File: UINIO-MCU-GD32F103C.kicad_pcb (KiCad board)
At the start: 2 copper layers, 68.4 x 20.3 mm, 41 parts, among them J1 Conn_01x24_Pin, J2 Conn_01x24_Pin, J3 Conn_01x04_Pin, SW1 BOOT1, SW2 NRST, SW3 BOOT0, U1 ME6211C33M5G-N, U2 GD32F103C8T6, Y1 32.768KHz, Y2 8MHz

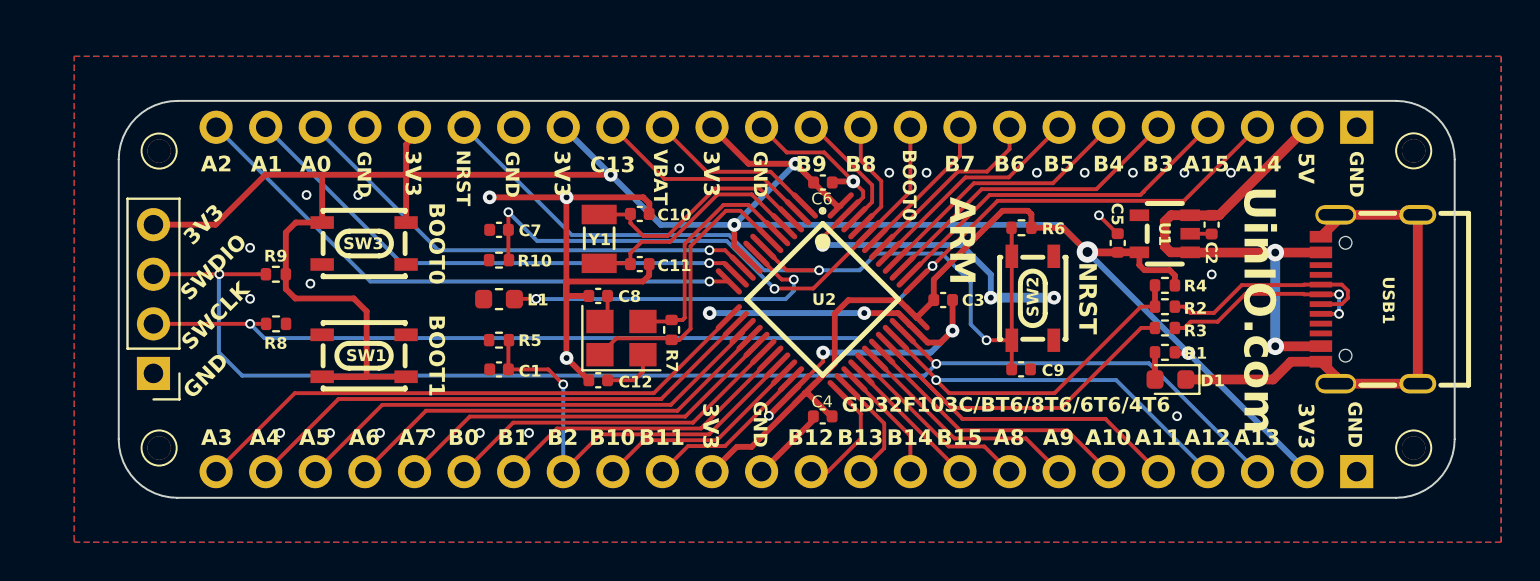
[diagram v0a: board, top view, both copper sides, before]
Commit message: Release UINIO-MCU-GD32F103C version 2.0.0.
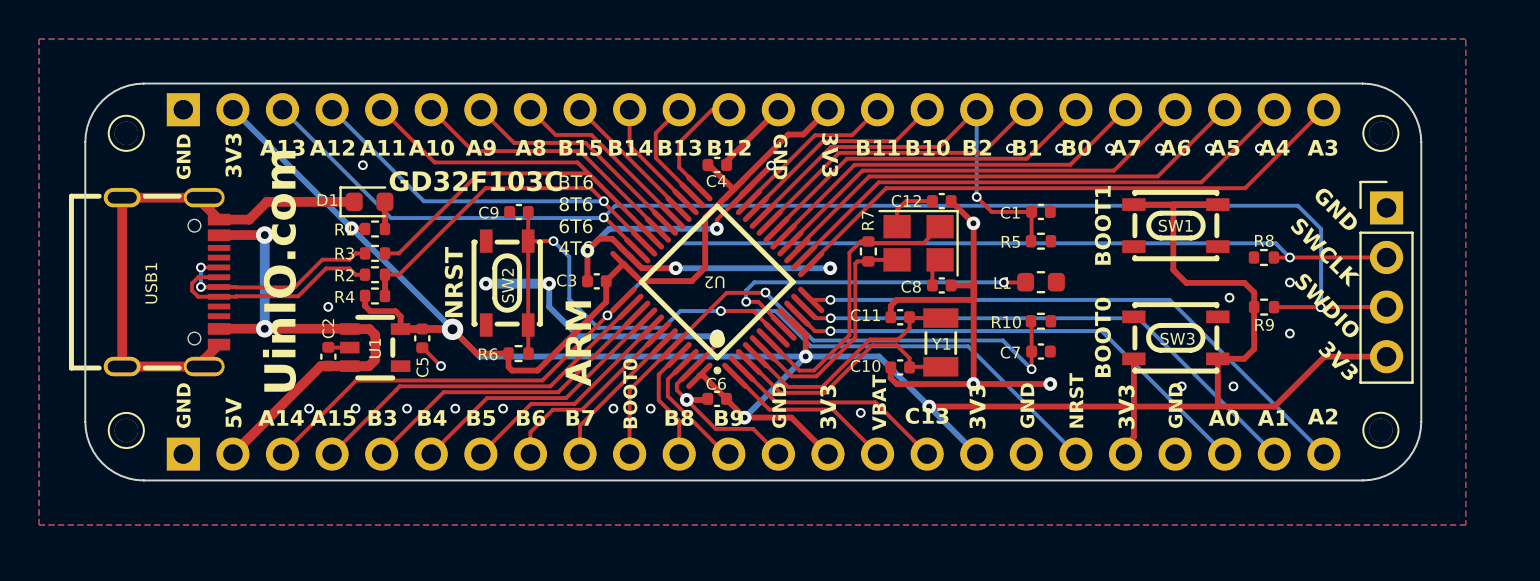
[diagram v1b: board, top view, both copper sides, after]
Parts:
- moved HOLE** 67.9 mm to (119.4, 92.2), turned to 180 degrees
- moved HOLE** 67.5 mm to (119.4, 107.4), turned to 180 degrees
- moved HOLE** 64.6 mm to (183.7, 92.2), turned to 180 degrees
- moved HOLE** 64.2 mm to (183.7, 107.4), turned to 180 degrees
- moved J3 63.7 mm to (184.0, 96.0), turned to 0 degrees
- moved J1 62.9 mm to (122.3, 91.0), turned to -90 degrees
- moved J2 62.4 mm to (122.3, 108.7), turned to -90 degrees
- moved USB1 61.4 mm to (121.7, 99.8), turned to -90 degrees
- moved R8 50.7 mm to (177.7, 98.6), turned to 0 degrees
- moved R9 50.6 mm to (177.7, 101.1), turned to 180 degrees
- moved C2 45.7 mm to (129.8, 103.7), turned to -90 degrees
- moved SW1 42.1 mm to (173.2, 96.9), turned to 180 degrees
- moved D1 42.0 mm to (131.9, 95.7), turned to 0 degrees
- moved SW3 41.9 mm to (173.2, 102.7), turned to 0 degrees
- moved R1 41.0 mm to (132.1, 97.1), turned to 180 degrees
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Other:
- board text added: "BT6 8T6 6T6 4T6"
- board text added: "GD32F103C"
- board text removed: "GD32F103C/BT6/8T6/6T6/4T6"
